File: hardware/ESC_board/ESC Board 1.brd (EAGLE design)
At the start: 90.8 x 78.7 mm, 15 parts

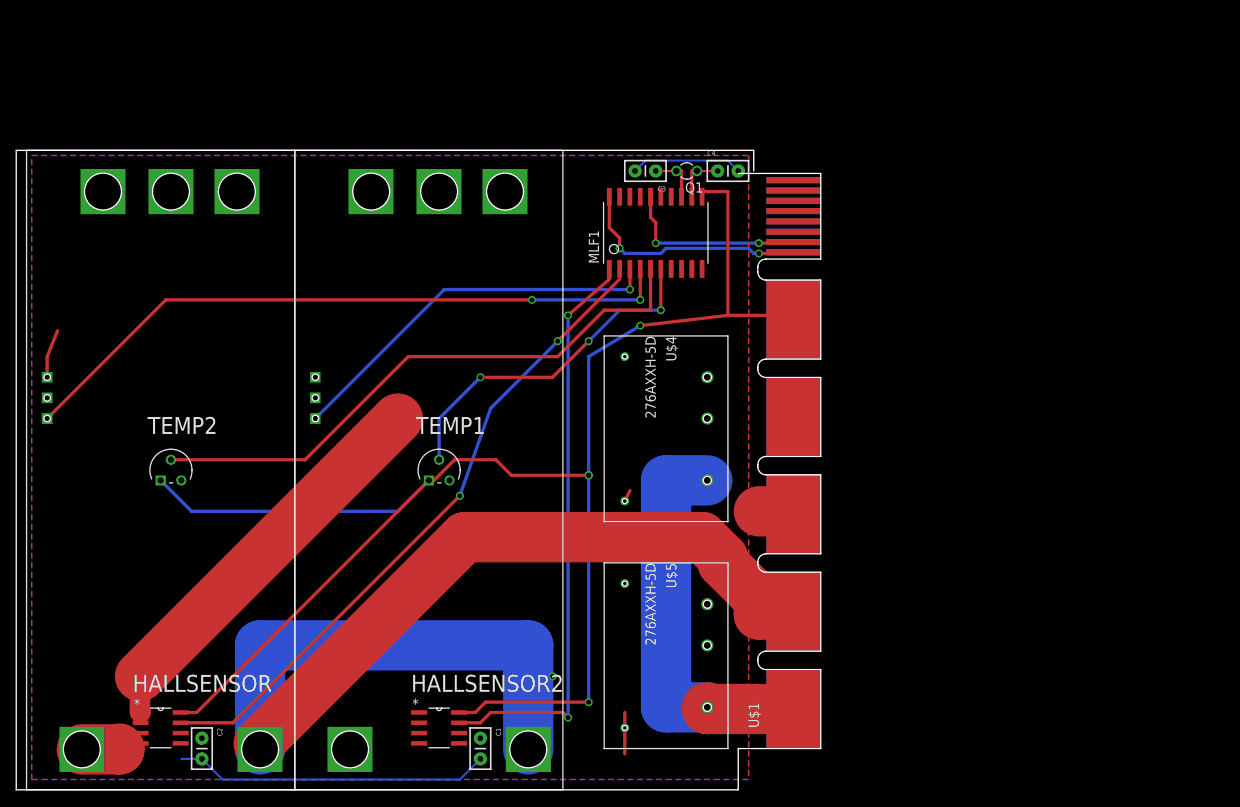
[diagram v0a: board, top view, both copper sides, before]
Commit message: total redesign is way better
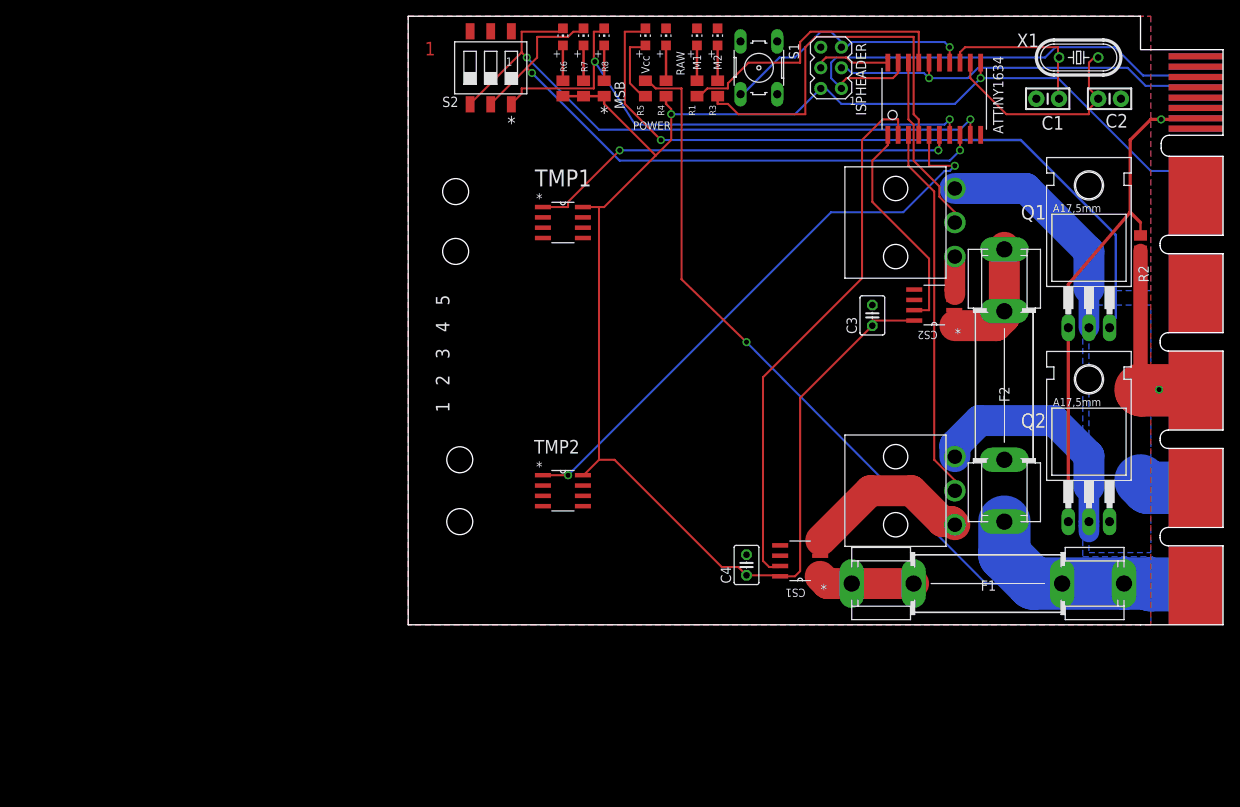
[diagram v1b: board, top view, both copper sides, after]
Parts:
- removed C2: (no value), SparkFun-Capacitors:CAP-PTH-SMALLEZ
- removed HALLSENSOR, HALLSENSOR2: ACS712ELCTR-20A-T, Allegro_By_element14_Batch_1:SOIC127P600X175-8N
- removed MLF1: ATTINY1634SOIC20, attiny1634:SOIC20
- removed TEMP1, TEMP2: TMP36GT9Z, ADI-Phase-2:TO127P254X533-3P
- removed U$4, U$5: 276AXXH-5D, Schneider Relay:276AXXH-5D
- added ATTINY1634: ATTINY1634SOIC20, attiny1634:SOIC20
- added BATTERIES, TMP1: TMP36GSZ, ADI-Phase-2:SOIC127P600X175-8N
- added C5: (no value), SparkFun-Capacitors:CAP-PTH-SMALL-KIT
- added CS1, CS2: ACS712ELCTR-20A-T, Allegro_By_element14_Batch_1:SOIC127P600X175-8N
- added F1, F2: FUSESH32, fuse:SH32
- added ISPHEADER: AVRISP-6, adafruit:AVRISP
- added LED1, LED2, LED3, LED4, LED5, LED7, LED8: (no value), adafruit:CHIP-LED0805
- added Q2: BUZ11, transistor-fet:TO220
- added Q3: (no value), crystal:HC49/S
- added R1, R2, R3, R4, R5, R6, R7, R8: (no value), adafruit:M2012
- added S1: (no value), switch-omron:B3F-10XX
- added S2: SWS003, smd-special:SMS-003
- C1: device SparkFun-Capacitors:CAP-PTH-SMALLEZ -> SparkFun-Capacitors:CAP-PTH-SMALL-KIT
- C3, C4: device SparkFun-Capacitors:CAP-PTH-SMALLEZ -> rcl:C025-030X050
- Q1: value (none) -> BUZ11; device crystal:TC26V -> transistor-fet:TO220
- U$2, U$3: value ESC30A -> 1-ROW-3; device ESC-30A:30AESC -> con-molex-mini-fit:1-ROW
- moved C1 105.3 mm to (127.0, 85.1), turned to 180 degrees
- moved U$2 96.6 mm to (115.6, 36.8)
- moved U$3 69.9 mm to (115.6, 69.8)
- moved U$1 51.8 mm to (148.6, 20.3)
- moved Q1 51.2 mm to (132.1, 63.2), turned to 0 degrees
- moved C4 48.6 mm to (89.9, 27.7), turned to 90 degrees
- moved C3 32.1 mm to (105.4, 58.4), turned to 90 degrees
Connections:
- removed net BAT-: U$1.P9, U$2.GROUND, U$3.GROUND
- new net N$18: ATTINY1634.20, ISPHEADER.4
- new net N$20: ATTINY1634.13, C1.1, Q3.2
- new net N$21: LED5.A, R7.2
- new net N$22: ATTINY1634.6, TMP1.1
- new net N$23: LED4.A, R8.2
- new net N$24: ATTINY1634.3, U$2.2
- new net N$25: LED2.A, R5.1
- new net N$26: ATTINY1634.18, U$3.2
- new net N$27: LED8.A, R3.1
- new net N$28: LED7.A, R1.1
- new net N$32: LED1.A, R4.1
- new net N$35: CS1.1, CS1.2, F1.2A
- new net N$36: CS2.1, CS2.2, F2.2A
- new net VDD: F1.1A, F2.1A, R5.2, U$1.P5
- new net V_BATT: LED2.C, Q1.3, Q2.3, U$1.P4
- net GND: now also ATTINY1634.10, BATTERIES.4, C5.2, CS1.5, CS2.5, ISPHEADER.6, LED1.C, LED7.C, LED8.C, R2.1, S1.2, S2.1, S2.2, S2.3, TMP1.4, U$1.P3; no longer C2.2, HALLSENSOR.5, HALLSENSOR2.5, MLF1.10, TEMP1.3, TEMP2.3, U$1.P8, U$2.GNDS, U$3.GNDS, U$4.-COIL, U$5.-COIL
- net N$1: now also ATTINY1634.17, R1.2; no longer MLF1.5, TEMP2.2
- net N$10: now also ATTINY1634.5, BATTERIES.1; no longer HALLSENSOR2.3, HALLSENSOR2.4, U$3.VCC
- net N$11: now also ATTINY1634.7, LED4.C, S2.6; no longer U$1.P10, U$4.COM, U$5.COM
- net N$12: now also ATTINY1634.8, LED5.C, S2.5; no longer HALLSENSOR.3, HALLSENSOR.4, U$2.VCC
- net N$13: now also ATTINY1634.9, LED3.C, S2.4; no longer MLF1.4, U$2.SIGNALS
- net N$14: now also LED3.A, R6.2; no longer MLF1.3, U$3.SIGNALS
- net N$15: now also CS1.3, CS1.4, U$2.1; no longer C2.1, HALLSENSOR.6
- net N$16: now also ATTINY1634.16, ISPHEADER.3, U$1.S4; no longer HALLSENSOR.1, HALLSENSOR.2, U$4.NO
- net N$17: now also ATTINY1634.14, ISPHEADER.5, S1.4; no longer HALLSENSOR2.1, HALLSENSOR2.2, U$5.NO
- net N$19: now also ATTINY1634.12, C5.1, Q3.1; no longer U$1.S9, U$4.+COIL, U$5.+COIL
- net N$2: now also Q1.1, Q2.1, R2.2, U$1.S7; no longer MLF1.6, TEMP1.2
- net N$3: now also ATTINY1634.4, R3.2; no longer MLF1.20, U$1.S16
- net N$4: now also Q1.2, U$3.3; no longer MLF1.16, U$1.S15
- net N$5: now also Q2.2, U$2.3; no longer HALLSENSOR2.7, MLF1.1
- net N$6: now also ATTINY1634.19, ISPHEADER.1, U$1.S3; no longer HALLSENSOR.7, MLF1.2
- net N$7: now also CS2.3, CS2.4, U$3.1; no longer C3.1, MLF1.13, Q1.2
- net N$8: now also ATTINY1634.1, CS2.7; no longer C4.1, MLF1.12, Q1.1
- net N$9: now also ATTINY1634.2, CS1.7; no longer C1.1, HALLSENSOR2.6
- net VCC: now also ATTINY1634.11, BATTERIES.8, C3.1, C4.1, CS1.8, CS2.8, ISPHEADER.2, R4.2, R6.1, R7.1, R8.1, TMP1.8, U$1.P1; no longer HALLSENSOR.8, HALLSENSOR2.8, MLF1.11, TEMP1.1, TEMP2.1, U$1.P6
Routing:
- net BAT-: track 143.6 -> 0.00 mm, vias 1 -> 0
- net VDD: track 0.00 -> 127.1 mm, vias 0 -> 1
- net V_BATT: track 0.00 -> 97.8 mm, vias 0 -> 1
- net N$10: track 0.00 -> 73.5 mm, vias 0 -> 2
- net N$12: track 4.72 -> 77.6 mm, vias 0 -> 2
- net N$9: track 0.00 -> 66.7 mm
- net N$22: track 0.00 -> 53.9 mm, vias 0 -> 2
- net N$24: track 0.00 -> 46.2 mm
- net N$14: track 47.9 -> 4.35 mm, vias 1 -> 0
- net N$5: track 71.8 -> 30.4 mm, vias 2 -> 0
- net GND: track 69.5 -> 28.7 mm
- net N$1: track 71.8 -> 36.7 mm
- net N$17: track 0.00 -> 32.8 mm, vias 0 -> 1
- net N$19: track 0.00 -> 27.1 mm
- net N$2: track 43.0 -> 66.7 mm, vias 3 -> 1
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- added copper zone on layer 16, net V_BATT
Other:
- board size 90.8 x 78.7 mm -> 90.2 x 74.9 mm
- board text added: "*"
- board text added: "1"
- board text added: "1 2 3 4 5"
- board text added: "C1"
- board text added: "C2"
- board text added: "M1"
- board text added: "M2"
- board text added: "MSB"
- board text added: "POWER"
- board text added: "RAW"
- board text added: "TMP2"
- board text added: "Vcc"
- board text added: "X1"
